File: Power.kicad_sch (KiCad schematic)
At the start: 20 parts, among them IC1 LM74502HDDFR, J1 CarLVPowerConnector, J3 Conn_01x02, Q1 PSMN8R5-40MSDX

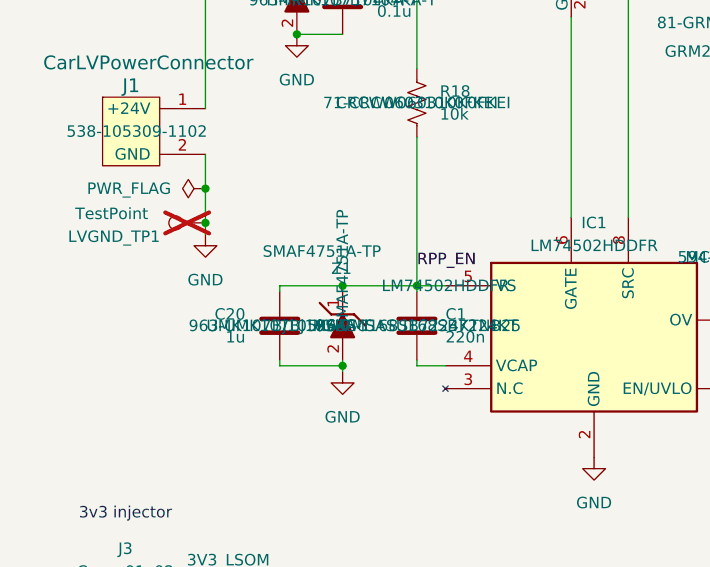
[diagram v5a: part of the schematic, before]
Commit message: alsdjflasjfsad
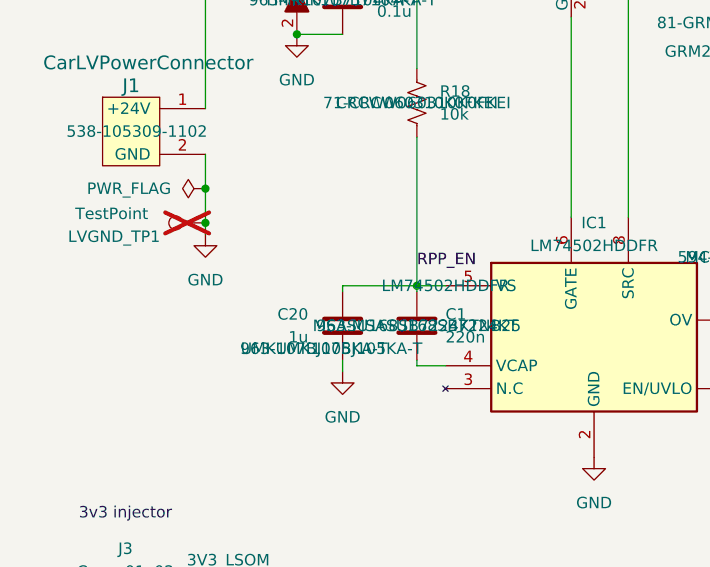
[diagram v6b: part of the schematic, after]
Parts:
- removed Z1: SMAF4751A-TP, UTSVT_Passives:SODFL5026X125N, symbol UTSVT_Power:SMAF4749A-TP
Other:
- moved on the sheet: C20
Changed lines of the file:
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@@
-	)
-	(junction
-		(at 62.865 77.47)
-		(diameter 0)
-		(color 0 0 0 0)
 	)
 	(junction
@@
 	)
 	(junction
-		(at 62.865 68.58)
-		(diameter 0)
-		(color 0 0 0 0)
-	)
-	(junction
 		(at 71.12 33.02)
 		(diameter 0)
@@
 	(wire
 		(pts
-			(xy 55.88 68.58) (xy 55.88 69.215)
-		)
-		(stroke
-			(width 0)
-			(type default)
-		)
-	)
-	(wire
-		(pts
-			(xy 55.88 68.58) (xy 62.865 68.58)
-		)
-		(stroke
-			(width 0)
-			(type default)
-		)
-	)
-	(wire
-		(pts
 			(xy 62.865 68.58) (xy 62.865 69.215)
 		)
@@
 	(wire
 		(pts
-			(xy 55.88 77.47) (xy 62.865 77.47)
-		)
-		(stroke
-			(width 0)
-			(type default)
-		)
-	)
-	(wire
-		(pts
 			(xy 190.5 52.705) (xy 190.5 57.785)
 		)
@@
 	(wire
 		(pts
-			(xy 62.865 76.835) (xy 62.865 77.47)
-		)
-		(stroke
-			(width 0)
-			(type default)
-		)
-	)
-	(wire
-		(pts
-			(xy 62.865 77.47) (xy 62.865 78.105)
-		)
-		(stroke
-			(width 0)
-			(type default)
-		)
-	)
-	(wire
-		(pts
 			(xy 43.815 104.14) (xy 50.165 104.14)
 		)
@@
 	(wire
 		(pts
-			(xy 55.88 77.47) (xy 55.88 76.835)
+			(xy 62.865 76.835) (xy 62.865 78.105)
 		)
 		(stroke
@@
 	)
 	(symbol
-		(lib_id "UTSVT_Power:SMAF4749A-TP")
-		(at 62.865 66.675 270)
-		(unit 1)
-		(exclude_from_sim no)
-		(in_bom yes)
-		(on_board yes)
-		(dnp no)
-		(property "Reference" "Z1"
-			(at 61.595 66.675 90)
-			(effects
-				(font
-					(size 1.27 1.27)
-				)
-				(justify left)
-			)
-		)
-		(property "Value" "SMAF4751A-TP"
-			(at 53.975 64.77 90)
-			(effects
-				(font
-					(size 1.27 1.27)
-				)
-				(justify left)
-			)
-		)
-		(property "Footprint" "UTSVT_Passives:SODFL5026X125N"
-			(at -30.785 76.835 0)
-			(effects
-				(font
-					(size 1.27 1.27)
-				)
-				(justify left top)
-				(hide yes)
-			)
-		)
-		(property "Datasheet" "https://www.mccsemi.com/pdf/Products/SMAF4735A_SMAF4764A(DO-221AC).pdf"
-			(at -130.785 76.835 0)
-			(effects
-				(font
-					(size 1.27 1.27)
-				)
-				(justify left top)
-				(hide yes)
-			)
-		)
-		(property "Description" "1.0 Watt Zener Diodes 6.2V to 100V"
-			(at 62.865 66.675 0)
-			(effects
-				(font
-					(size 1.27 1.27)
-				)
-				(hide yes)
-			)
-		)
-		(property "Height" "1.25"
-			(at -330.785 76.835 0)
-			(effects
-				(font
-					(size 1.27 1.27)
-				)
-				(justify left top)
-				(hide yes)
-			)
-		)
-		(property "Mouser Part Number" "833-SMAF4749A-TP"
-			(at -430.785 76.835 0)
-			(effects
-				(font
-					(size 1.27 1.27)
-				)
-				(justify left top)
-				(hide yes)
-			)
-		)
-		(property "Mouser Price/Stock" "https://www.mouser.co.uk/ProductDetail/Micro-Commercial-Components-MCC/SMAF4749A-TP?qs=%252BXxaIXUDbq1bdSZ3Ebik%2FA%3D%3D"
-			(at -530.785 76.835 0)
-			(effects
-				(font
-					(size 1.27 1.27)
-				)
-				(justify left top)
-				(hide yes)
-			)
-		)
-		(property "Manufacturer_Name" "MCC"
-			(at -630.785 76.835 0)
-			(effects
-				(font
-					(size 1.27 1.27)
-				)
-				(justify left top)
-				(hide yes)
-			)
-		)
-		(property "Manufacturer_Part_Number" "SMAF4749A-TP"
-			(at -730.785 76.835 0)
-			(effects
-				(font
-					(size 1.27 1.27)
-				)
-				(justify left top)
-				(hide yes)
-			)
-		)
-		(property "P/N" "SMAF4751A-TP"
-			(at 62.865 66.675 0)
-			(effects
-				(font
-					(size 1.27 1.27)
-				)
-			)
-		)
-		(pin "1"
-		)
-		(pin "2"
-		)
-		(instances
-			(project "VehicleControlUnit"
-				(path "/795c8e51-3ded-4d21-b864-aaff31c5def7/5469fc22-573e-4402-96df-d8b4b5bb4d29"
-					(reference "Z1")
-					(unit 1)
-				)
-			)
-		)
-	)
-	(symbol
 		(lib_id "Device:C")
 		(at 216.535 45.085 0)
@@
 	(symbol
 		(lib_id "Device:C")
-		(at 55.88 73.025 0)
+		(at 62.865 73.025 0)
 		(mirror x)
 		(unit 1)
@@
 		(on_board yes)
 		(dnp no)
-		(fields_autoplaced yes)
 		(property "Reference" "C20"
-			(at 52.07 71.7549 0)
+			(at 59.055 71.7549 0)
 			(effects
 				(font
@@
 		)
 		(property "Value" "1u"
-			(at 52.07 74.2949 0)
+			(at 59.055 74.2949 0)
 			(effects
 				(font
@@
 		)
 		(property "Footprint" "Capacitor_SMD:C_0603_1608Metric"
-			(at 56.8452 69.215 0)
+			(at 63.8302 69.215 0)
 			(effects
 				(font
@@
 		)
 		(property "Datasheet" "~"
-			(at 55.88 73.025 0)
+			(at 62.865 73.025 0)
 			(effects
 				(font
@@
 		)
 		(property "Description" "Unpolarized capacitor"
-			(at 55.88 73.025 0)
+			(at 62.865 73.025 0)
 			(effects
 				(font
@@
 		)
 		(property "P/N" "UMK107BJ105KA-T"
-			(at 55.88 73.025 0)
+			(at 59.69 75.565 0)
 			(effects
 				(font
@@
 		)
 		(property "Mouser Part Number" "963-UMK107BJ105KA-T"
-			(at 55.88 73.025 0)
-			(effects
-				(font
+			(at 61.595 75.565 0)
+			(effects
+				(font

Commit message: workday
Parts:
- C1, C19, C20, C4, C5: footprint Capacitor_SMD:C_0603_1608Metric -> Capacitor_SMD:C_0603_1608Metric_Pad1.08x0.95mm_HandSolder
- C21, C3: footprint Capacitor_SMD:C_0805_2012Metric -> Capacitor_SMD:C_0805_2012Metric_Pad1.18x1.45mm_HandSolder
- R1, R13, R18, R28: footprint Resistor_SMD:R_0603_1608Metric -> Resistor_SMD:R_0603_1608Metric_Pad0.98x0.95mm_HandSolder
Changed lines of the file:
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@@
 			)
 		)
-		(property "Footprint" "Capacitor_SMD:C_0603_1608Metric"
+		(property "Footprint" "Capacitor_SMD:C_0603_1608Metric_Pad1.08x0.95mm_HandSolder"
 			(at 70.1548 76.835 0)
 			(effects
@@
 			)
 		)
-		(property "Footprint" "Resistor_SMD:R_0603_1608Metric"
+		(property "Footprint" "Resistor_SMD:R_0603_1608Metric_Pad0.98x0.95mm_HandSolder"
 			(at 72.136 48.514 90)
 			(effects
@@
 			)
 		)
-		(property "Footprint" "Capacitor_SMD:C_0603_1608Metric"
+		(property "Footprint" "Capacitor_SMD:C_0603_1608Metric_Pad1.08x0.95mm_HandSolder"
 			(at 227.6602 48.895 0)
 			(effects
@@
 			)
 		)
-		(property "Footprint" "Capacitor_SMD:C_0603_1608Metric"
+		(property "Footprint" "Capacitor_SMD:C_0603_1608Metric_Pad1.08x0.95mm_HandSolder"
 			(at 63.8302 40.64 0)
 			(effects
@@
 			)
 		)
-		(property "Footprint" "Capacitor_SMD:C_0603_1608Metric"
+		(property "Footprint" "Capacitor_SMD:C_0603_1608Metric_Pad1.08x0.95mm_HandSolder"
 			(at 217.5002 48.895 0)
 			(effects
@@
 			)
 		)
-		(property "Footprint" "Resistor_SMD:R_0603_1608Metric"
+		(property "Footprint" "Resistor_SMD:R_0603_1608Metric_Pad0.98x0.95mm_HandSolder"
 			(at 191.516 40.259 90)
 			(effects
@@
 			)
 		)
-		(property "Footprint" "Capacitor_SMD:C_0805_2012Metric"
+		(property "Footprint" "Capacitor_SMD:C_0805_2012Metric_Pad1.18x1.45mm_HandSolder"
 			(at 110.1852 43.18 0)
 			(effects
@@
 			)
 		)
-		(property "Footprint" "Resistor_SMD:R_0603_1608Metric"
+		(property "Footprint" "Resistor_SMD:R_0603_1608Metric_Pad0.98x0.95mm_HandSolder"
 			(at 120.904 71.374 90)
 			(effects
@@
 			)
 		)
-		(property "Footprint" "Capacitor_SMD:C_0603_1608Metric"
+		(property "Footprint" "Capacitor_SMD:C_0603_1608Metric_Pad1.08x0.95mm_HandSolder"
 			(at 63.8302 69.215 0)
 			(effects
@@
 			)
 		)
-		(property "Footprint" "Capacitor_SMD:C_0805_2012Metric"
+		(property "Footprint" "Capacitor_SMD:C_0805_2012Metric_Pad1.18x1.45mm_HandSolder"
 			(at 204.8002 48.895 0)
 			(effects
@@
 			)
 		)
-		(property "Footprint" "Resistor_SMD:R_0603_1608Metric"
+		(property "Footprint" "Resistor_SMD:R_0603_1608Metric_Pad0.98x0.95mm_HandSolder"
 			(at 112.141 65.659 90)
 			(effects

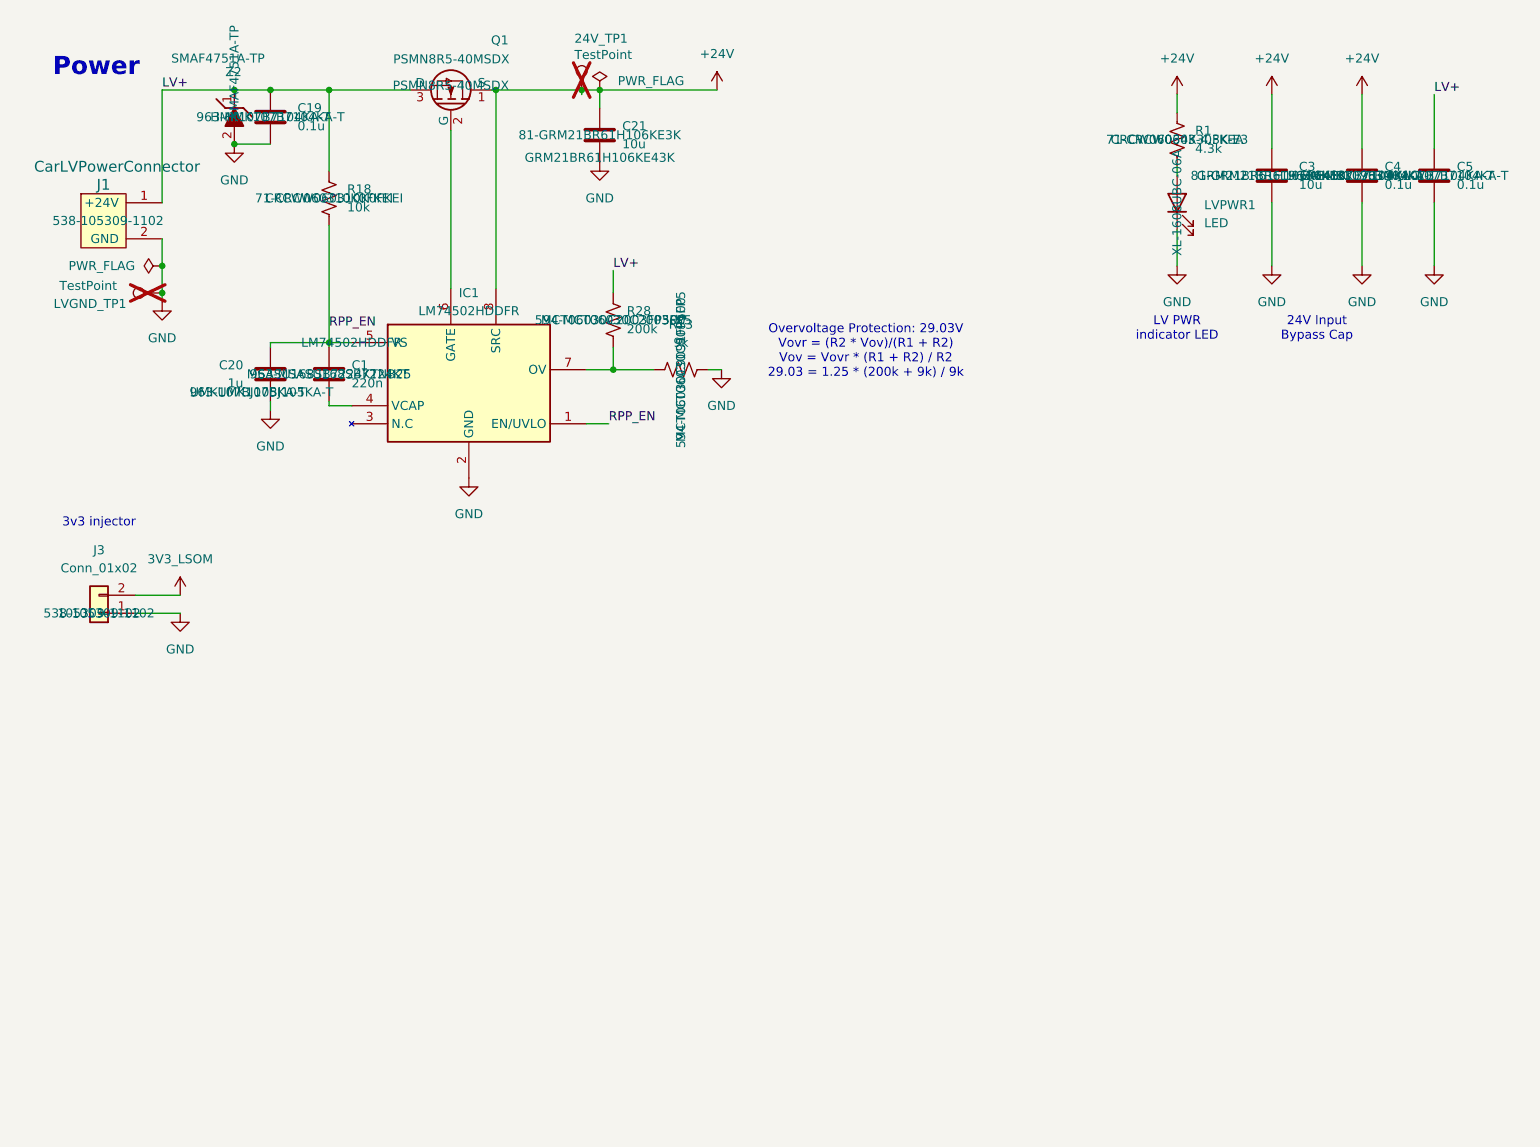
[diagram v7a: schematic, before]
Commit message: rev B
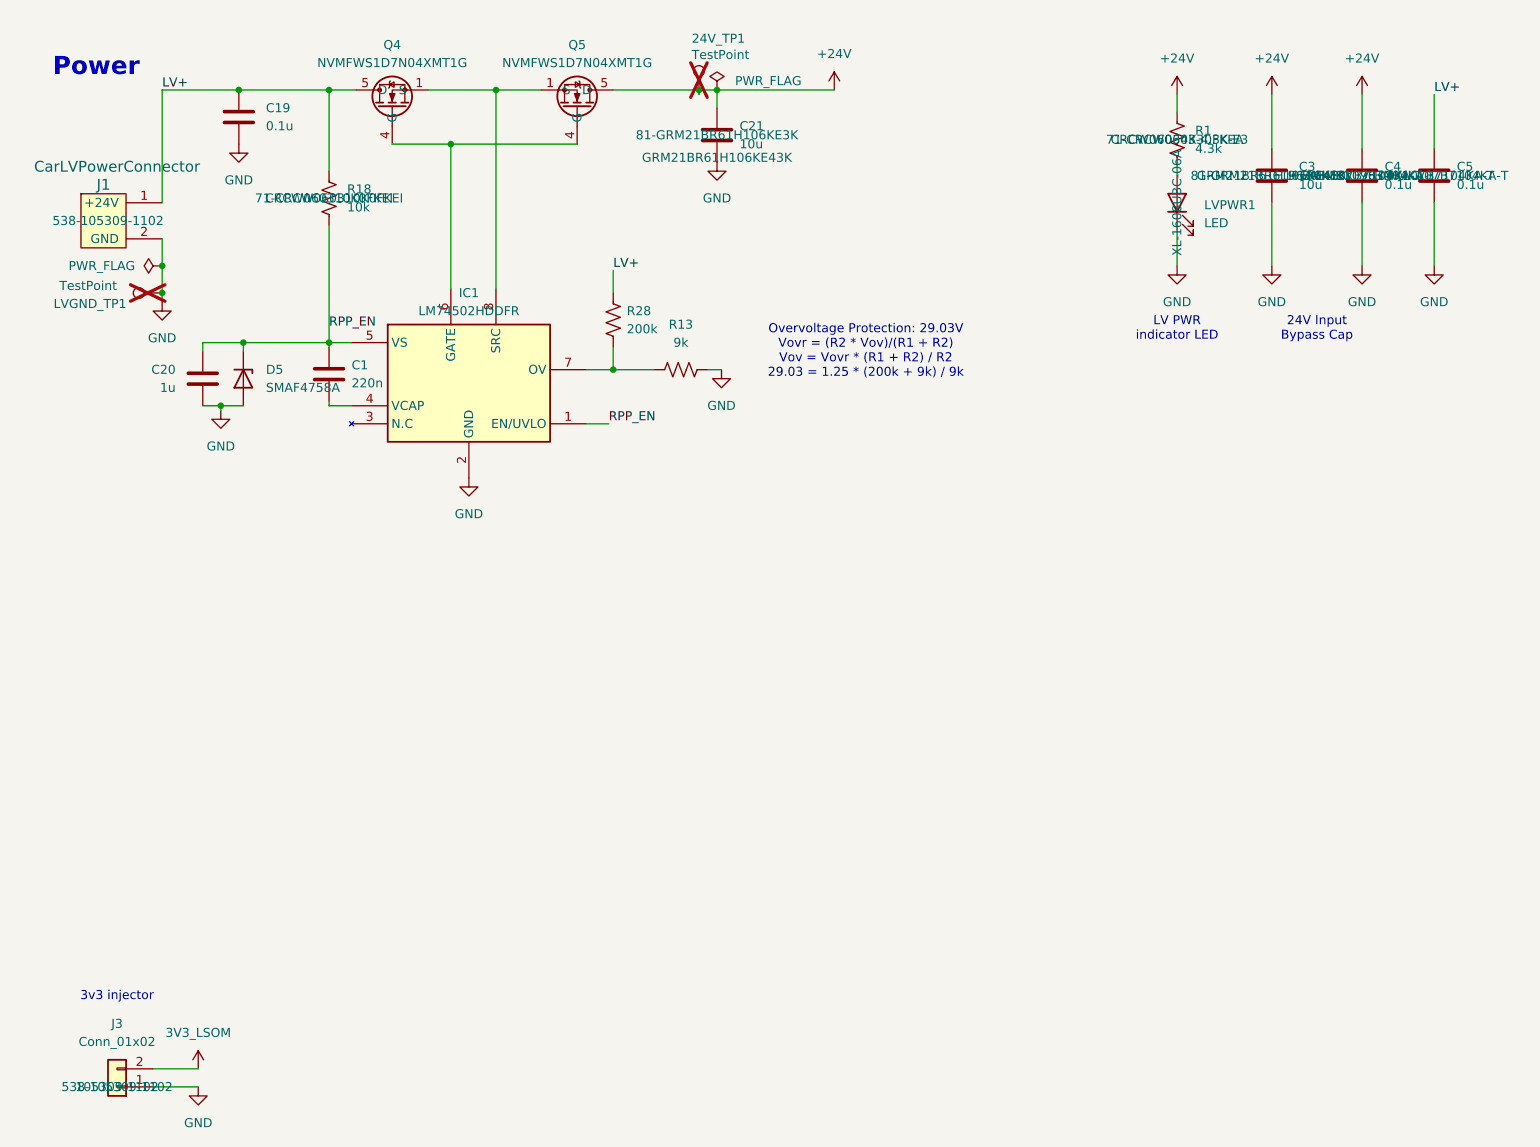
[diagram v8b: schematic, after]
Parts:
- removed Q1: PSMN8R5-40MSDX, UTSVT_Power:PSMN8R5-40MSDX, symbol UTSVT_Power:PSMN8R5-40MSDX
- removed Z2: SMAF4751A-TP, UTSVT_Passives:SODFL5026X125N, symbol UTSVT_Power:SMAF4749A-TP
- added D5: SMAF4758A, UTSVT_Passives:SODFL5026X125N, symbol Device:D_Zener
- added Q4, Q5: NVMFWS1D7N04XMT1G, UTSVT_Power:NVMFWS3D0P04M8LT1G, symbol UTSVT_Power:NVMFWS1D7N04XMT1G
- 24V_TP1, LVGND_TP1: footprint UTSVT_Special:TestPoint_HEX_3mmID -> TestPoint:TestPoint_Pad_2.0x2.0mm
- LVPWR1: footprint LED_SMD:LED_0603_1608Metric -> LED_SMD:LED_0603_1608Metric_Pad1.05x0.95mm_HandSolder
- R18: footprint Resistor_SMD:R_0603_1608Metric_Pad0.98x0.95mm_HandSolder -> Resistor_SMD:R_0805_2012Metric_Pad1.20x1.40mm_HandSolder
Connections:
- net +24V: now also Q5.5 (D), Q5.6 (D), Q5.7 (D), Q5.8 (D), Q5.9 (D); no longer IC1.8 (SRC)
- net GND: now also D5.2 (A)
- net LV+: now also Q4.5 (D), Q4.6 (D), Q4.7 (D), Q4.8 (D), Q4.9 (D)
- net RPP_EN: now also D5.1 (K)
- net at IC1.6 (GATE): now also Q4.4 (G), Q5.4 (G)
- new net: IC1.8 (SRC), Q4.1 (S), Q4.2 (S), Q4.3 (S), Q5.1 (S), Q5.2 (S), Q5.3 (S)
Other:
- moved on the sheet: 24V_TP1, C19, C20, C21, J3
